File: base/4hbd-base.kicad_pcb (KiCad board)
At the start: 2 copper layers, 150 x 100 mm, 198 parts, among them J1 Screw_Terminal_01x03, J10 Conn_01x08, J12 Spring_Terminal_Connector_01x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, J14 Screw_Terminal_01x02, J15 Conn_01x27, J16 Conn_01x27, J2 Screw_Terminal_01x03, J3 Screw_Terminal_01x03, J4 Screw_Terminal_01x03, J5 Screw_Terminal_01x02, J6 Screw_Terminal_01x02, J7 Screw_Terminal_01x02, J8 Screw_Terminal_01x02, J9 Screw_Terminal_01x04, Q1 irf540n, Q10 2N7002, Q11 2N7002, Q12 IRLML2060TRPBF, Q2 irf540n, Q3 irf540n, Q4 irf540n, Q5 irf540n, Q6 irf540n, Q7 irf540n, Q8 irf540n, U1 SI8640, U11 MOCD217M, U12 MOCD217M, U13 MOCD217M, U14 AMS1117-5.0, U15 AMS1117-5.0, U16 LM2596S-ADJ, U17 AM26LV32, U18 LM2596S-ADJ, U19 AMS1117-5.0, U2 SI8640, U3 IR25606, U4 IR25606, U5 IR25606, U6 IR25606, U7 ACS712xLCTR-30A, U8 ACS712xLCTR-30A

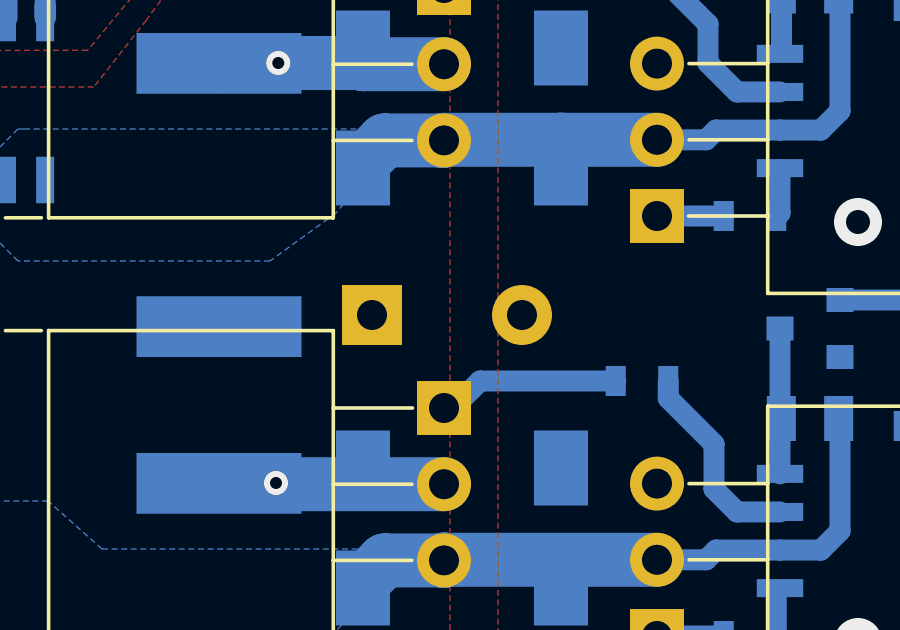
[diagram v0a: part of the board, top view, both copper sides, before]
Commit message: update gerbers
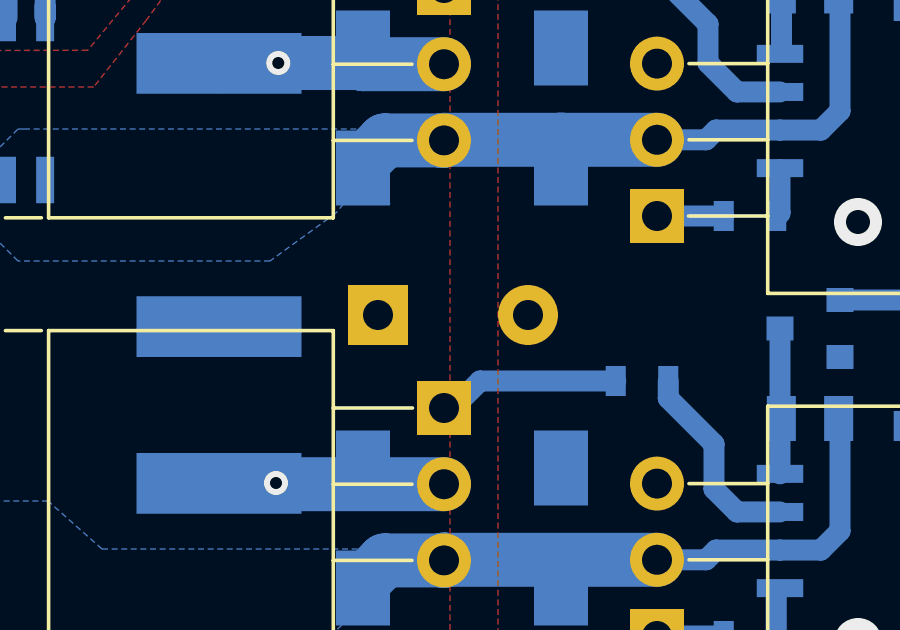
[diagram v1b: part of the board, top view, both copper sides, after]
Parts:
- moved C49 0.20 mm to (117.4, 102.0)
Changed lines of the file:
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@@
     (links 447)
     (no_connects 16)
-    (area 69.924999 62.924999 220.075001 163.075001)
+    (area 58.214287 62.625 220.075001 163.3)
     (thickness 1.6)
     (drawings 50)
@@
   (page A4)
   (layers
-    (0 F.Cu mixed hide)
-    (31 B.Cu mixed)
+    (0 F.Cu mixed)
+    (31 B.Cu mixed hide)
     (32 B.Adhes user hide)
     (33 F.Adhes user hide)
@@
     (visible_elements FFFEFF7F)
     (pcbplotparams
-      (layerselection 0x00030_80000001)
+      (layerselection 0x010f0_80000001)
       (usegerberextensions false)
+      (gerberprecision 5)
       (excludeedgelayer true)
       (linewidth 0.100000)
@@
       (viasonmask false)
       (mode 1)
-      (useauxorigin false)
+      (useauxorigin true)
       (hpglpennumber 1)
       (hpglpenspeed 20)
@@
       (psa4output false)
       (plotreference true)
-      (plotvalue true)
+      (plotvalue false)
       (plotinvisibletext false)
       (padsonsilk false)
@@
       (outputformat 1)
       (mirror false)
-      (drillshape 1)
+      (drillshape 0)
       (scaleselection 1)
-      (outputdirectory ""))
+      (outputdirectory fab/))
   )
   (net 0 "")
@@
   )
   (module Capacitor_THT:CP_Radial_D10.0mm_P5.00mm (layer B.Cu)
-    (at 117.2 102)
+    (at 117.4 102)
     (descr "CP, Radial series, Radial, pin pitch=5.00mm, diameter=10mm, Electrolytic Capacitor")
     (tags "CP Radial series Radial pin pitch 5.00mm  diameter 10mm Electrolytic Capacitor")
